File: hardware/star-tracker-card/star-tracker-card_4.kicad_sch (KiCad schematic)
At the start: 27 parts, among them U1 RCLAMP0504FB, U7 OSD3358-512M-BSM, Y1 24MHz, Y2 ABS07-32.768KHZ-T

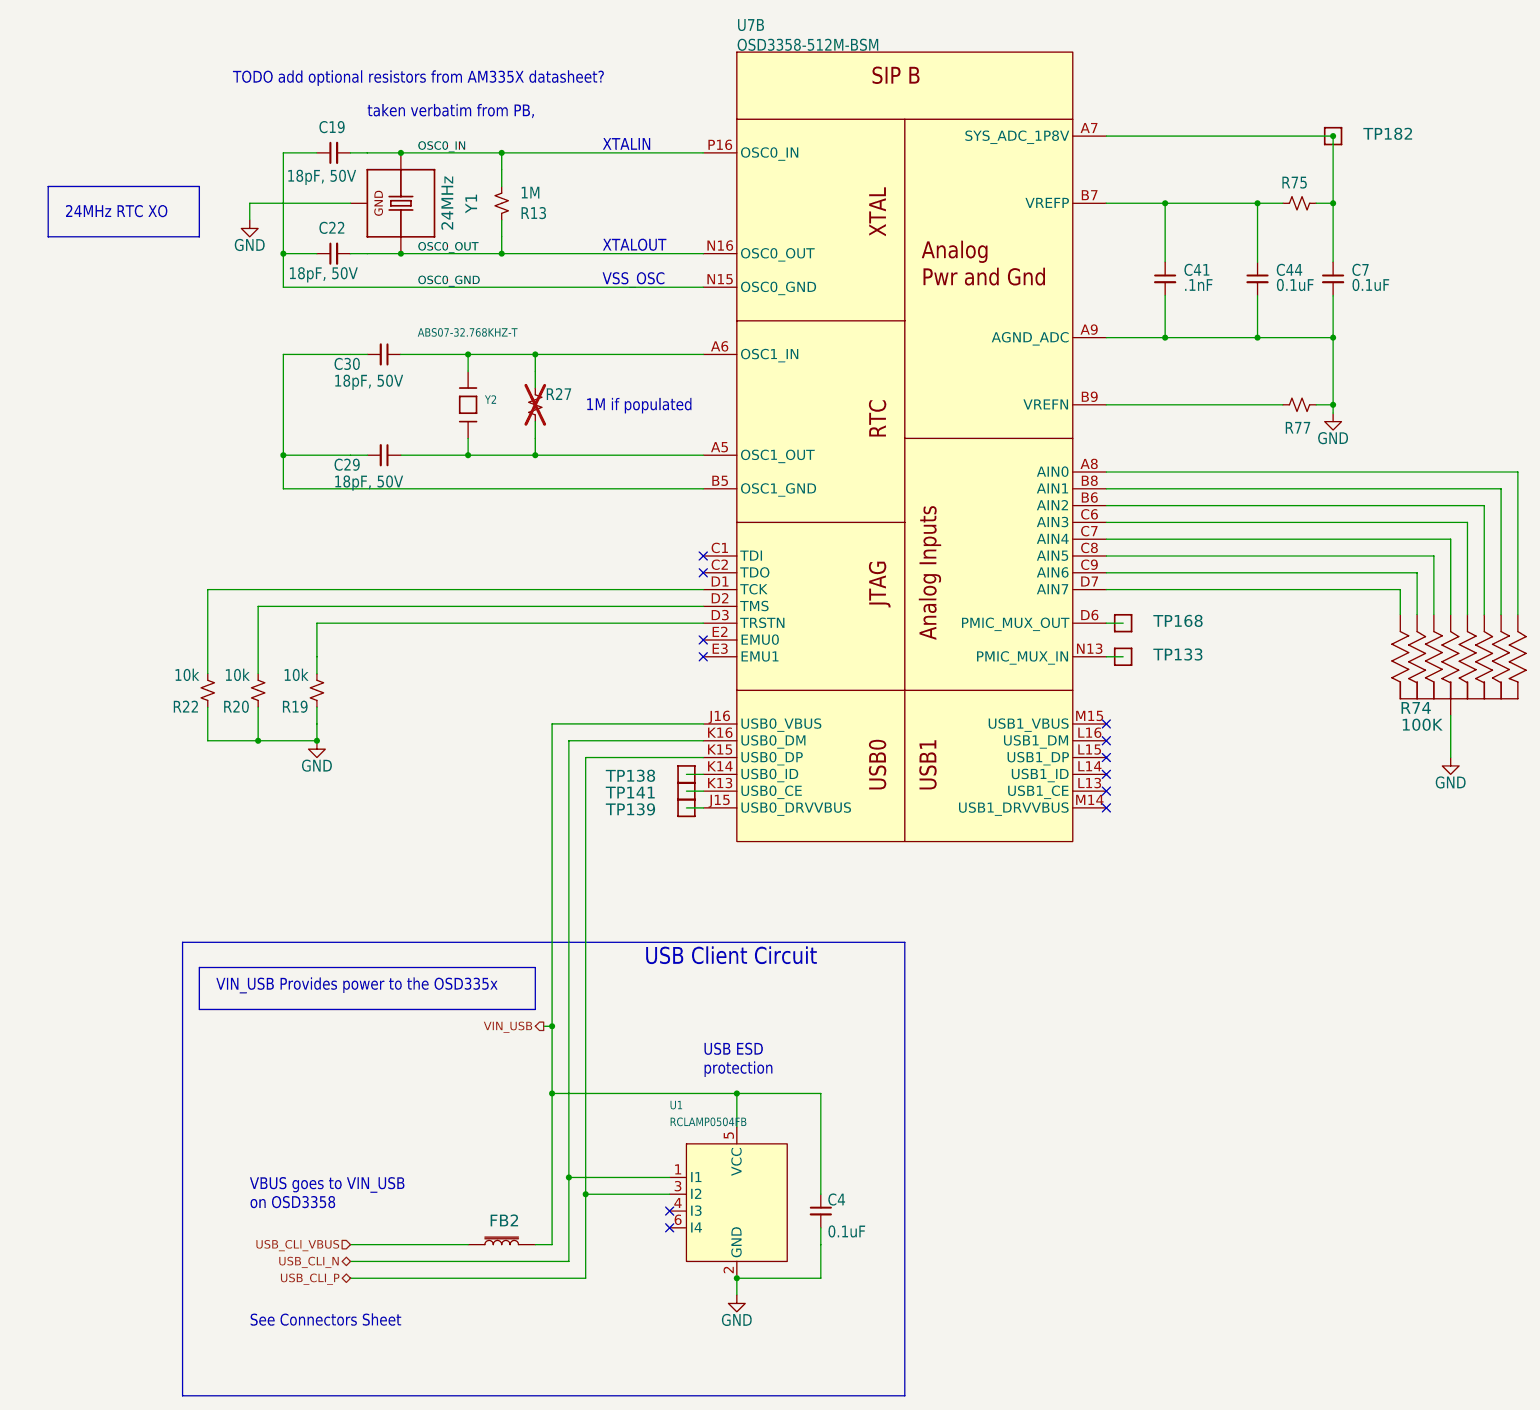
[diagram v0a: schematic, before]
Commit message: Update
Update to the octavo schematic
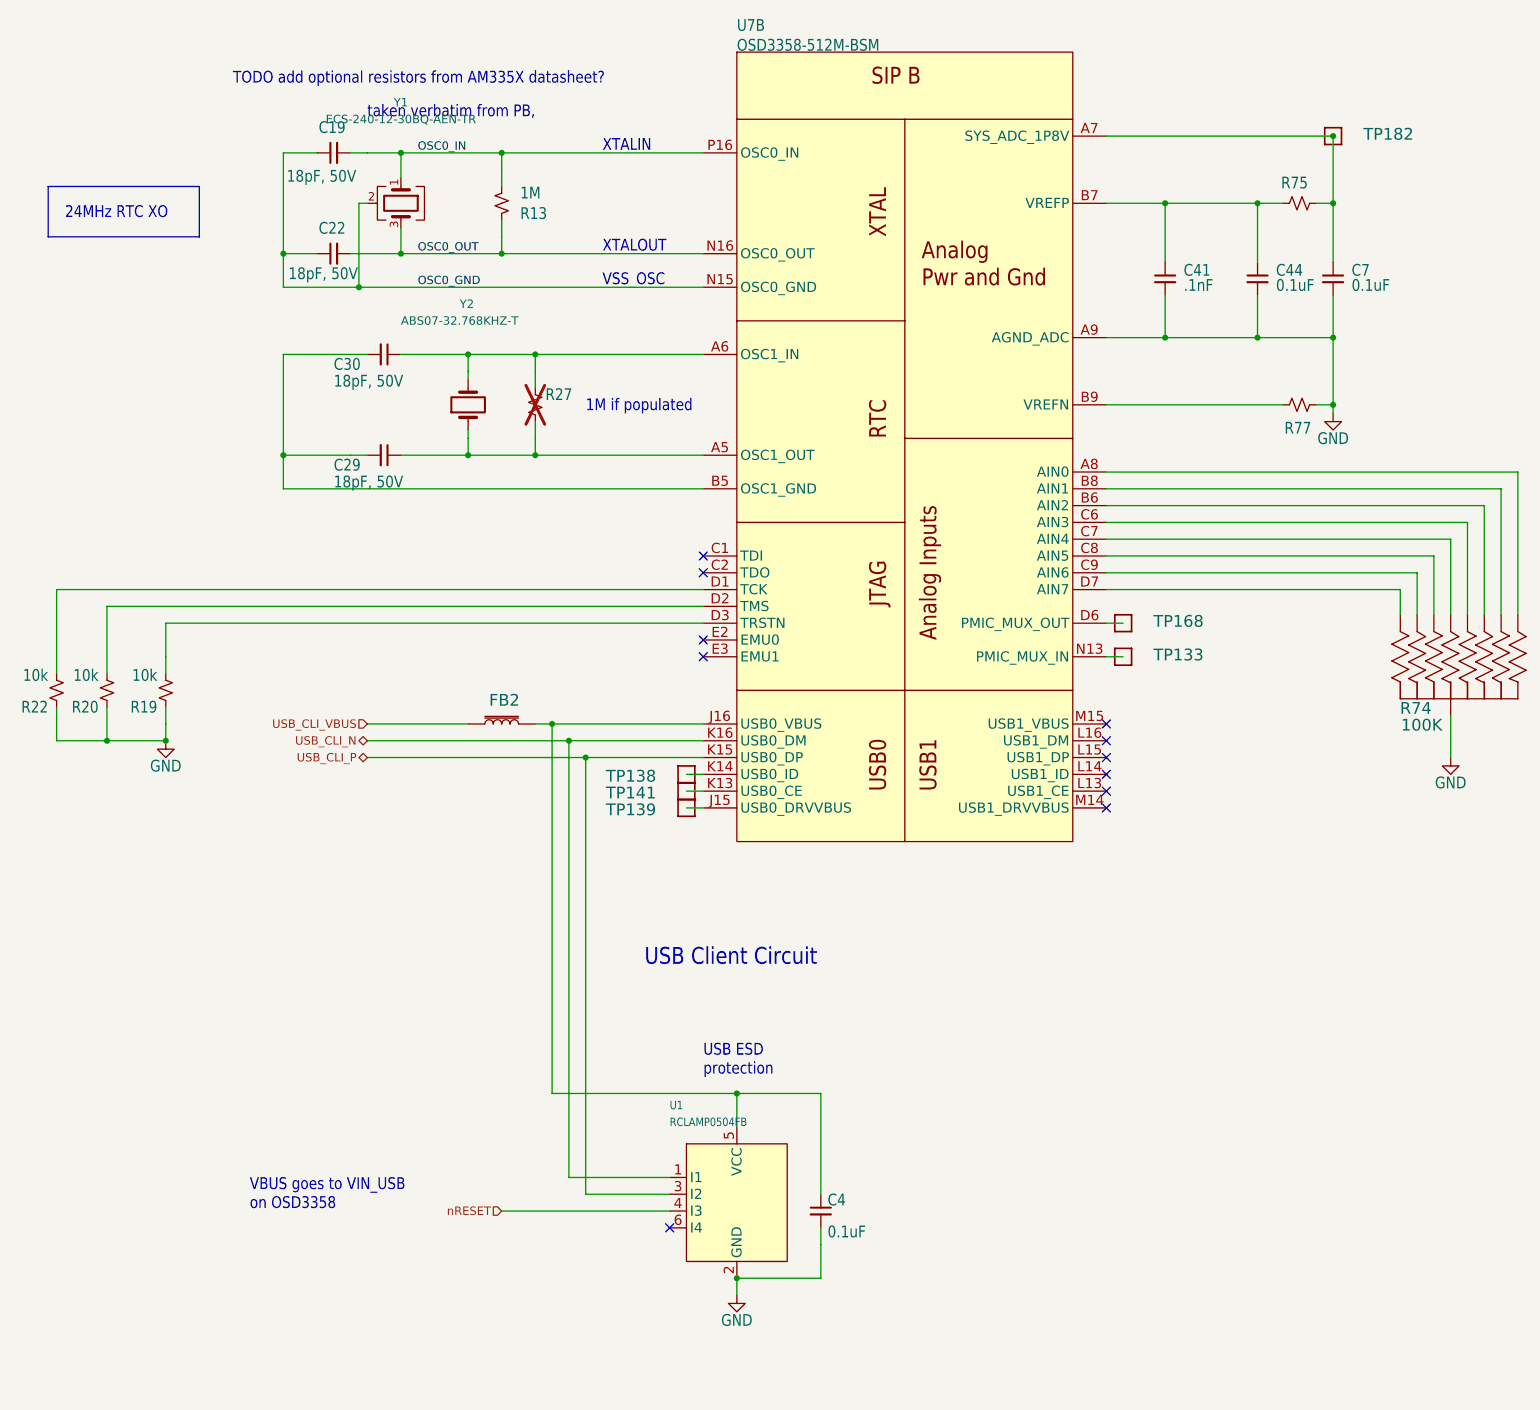
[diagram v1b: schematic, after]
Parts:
- removed Y1: 24MHz, star-tracker-card:5X3.2-4SMD, symbol star-tracker-card-eagle-import:ECS-240-12-30BQ-AEN-TR
- removed Y2: ABS07-32.768KHZ-T, star-tracker-card:CRYSTAL_3.2X1.5, symbol star-tracker-card-eagle-import:ABS07-32.768KHZ-T
- added Y1: ECS-240-12-30BQ-AEN-TR, oresat-passives:CRYSTAL-5X3.2-4SMD, symbol Device:Crystal_GND24
- added Y2: ABS07-32.768KHZ-T, oresat-passives:CRYSTAL_3.2X1.5, symbol Device:Crystal
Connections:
- net OSC0_GND: now also Y1.2 (G), Y1.4 (G)
- net OSC0_IN: now also Y1.1
- net OSC0_OUT: now also Y1.3
- net at C29.1, R27.1, U7.A5 (OSC1_OUT): now also Y2.1
- net at C30.1, R27.2, U7.A6 (OSC1_IN): now also Y2.2
- net nRESET: now reaches U1.4 (I3)
- net VIN_USB: no longer names the net of C4.1, FB2.2, U1.5 (VCC), U7.J16 (USB0_VBUS)
- no-connect marks 12 -> 11
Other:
- note removed: "See Connectors Sheet"
- note removed: "VIN_USB Provides power to the OSD335x"
- moved on the sheet: FB2, R19, R20, R22
